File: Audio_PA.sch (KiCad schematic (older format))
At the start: 71 parts, among them P1 Audio_In, P2 TP, P3 TP, P4 +45VDC, P5 Audio_Out, P6 -45VDC, Q1 BCM856DS, Q10 2N3904, Q11 2N3906, Q12 IRFP240, Q13 IRFP9240, Q2 BCM856DS, Q3 MJE340, Q4 MJE350, Q5 MJE350, Q6 MJE340, Q7 BD139, Q8 MJE340, Q9 MJE350

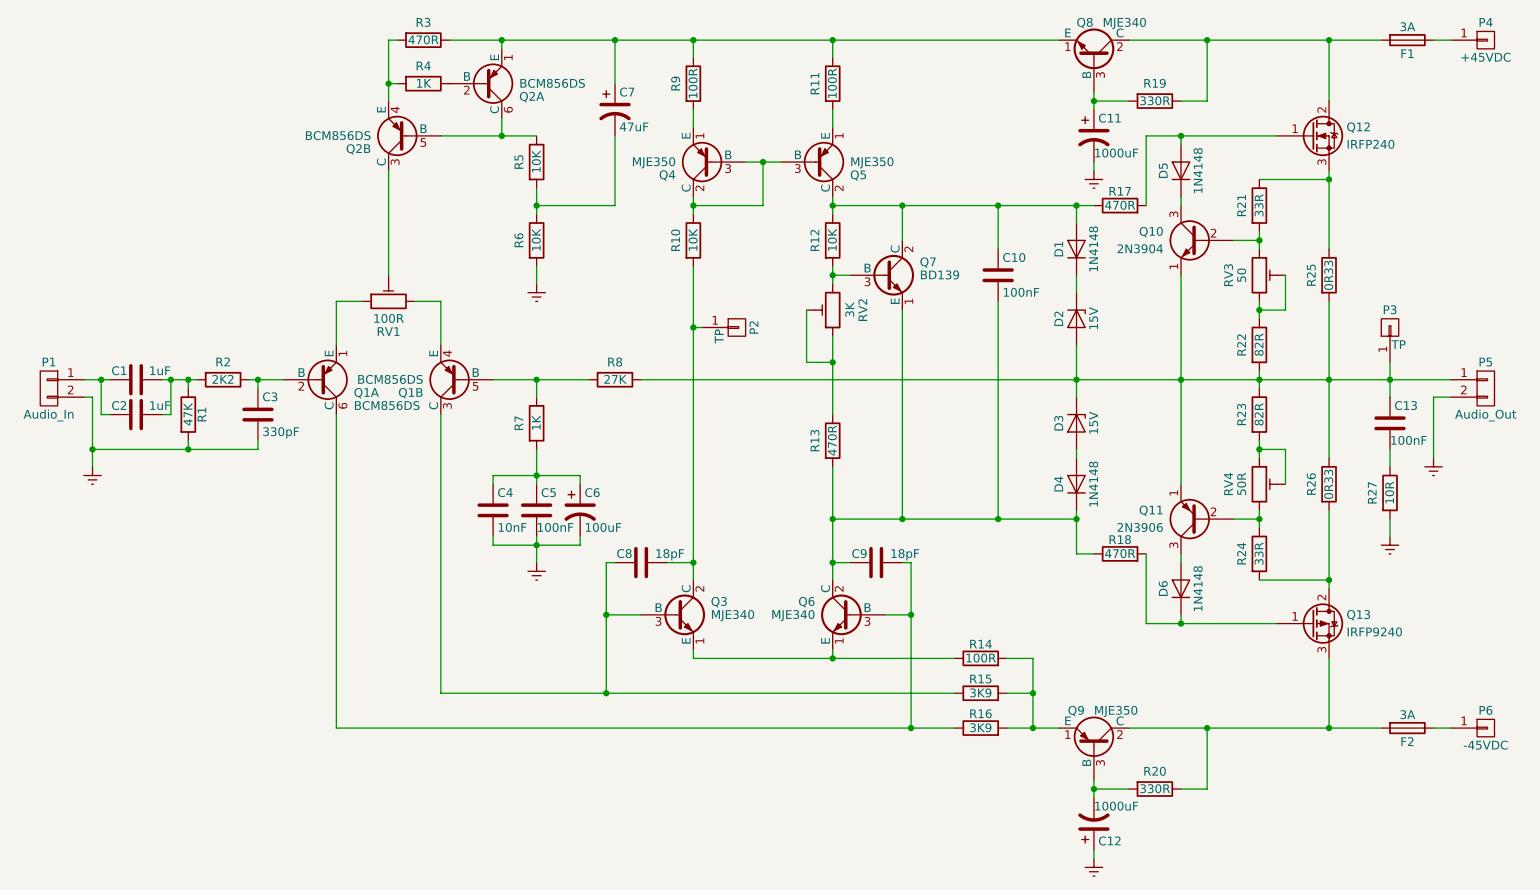
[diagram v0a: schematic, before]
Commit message: Layout V1 added
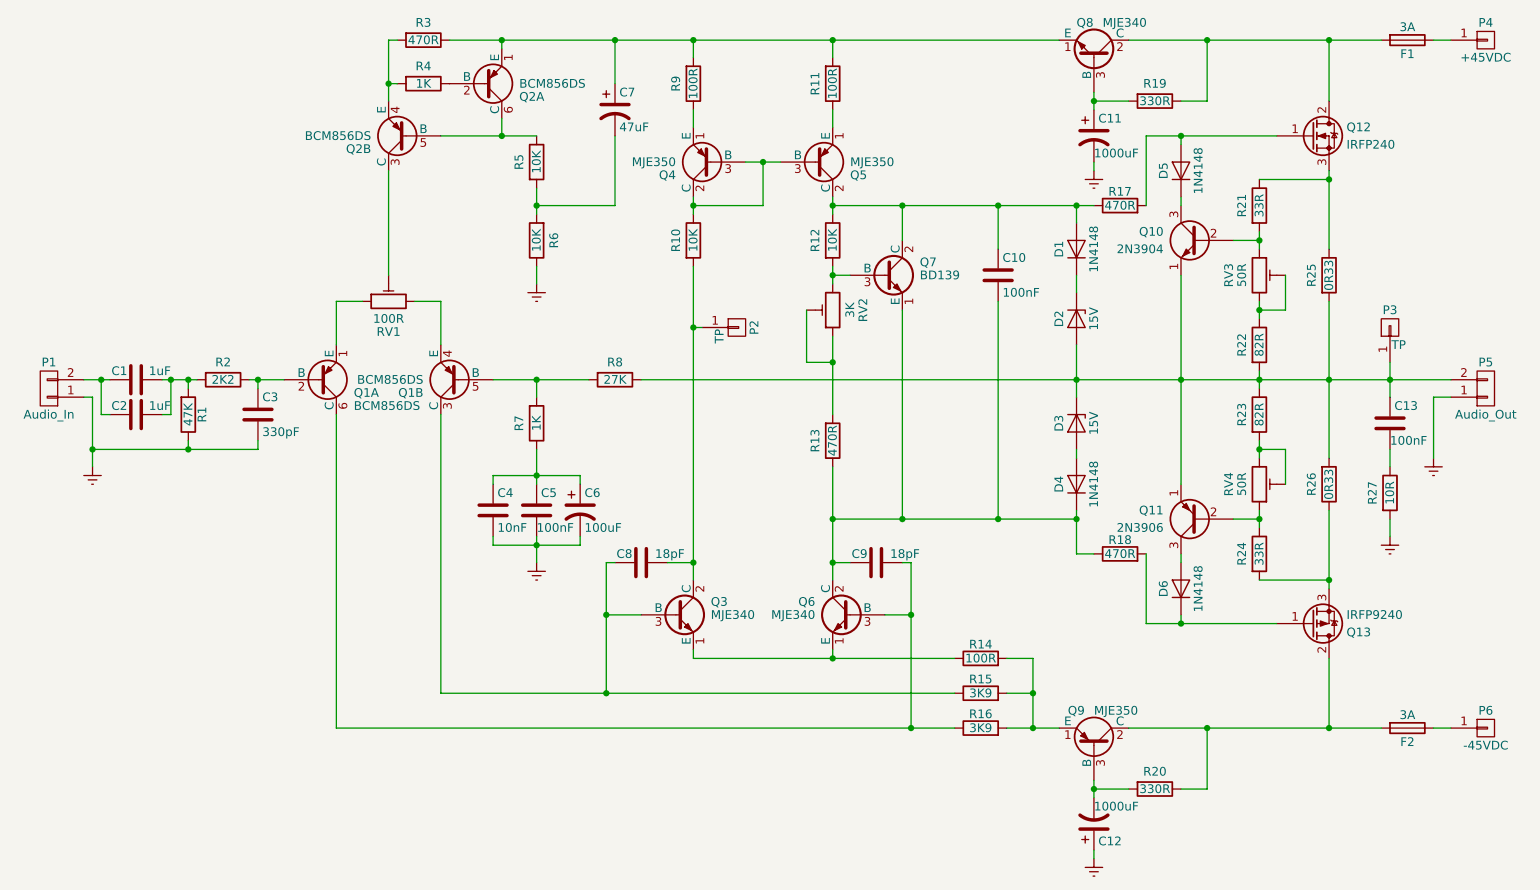
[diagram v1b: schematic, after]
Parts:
- Q7: footprint (none) -> TO_SOT_Packages_THT:SOT126_SOT32_Housing_Vertical
- RV3: value 50 -> 50R
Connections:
- net Earth: now also P1.1 (P1), P5.1 (P1), R1.1, R6.1; no longer P1.2 (P2), P5.2 (P2), R1.2, R6.2
- net at C1.1, C2.1: now also P1.2 (P2); no longer P1.1 (P1)
- net at C1.2, C2.2, R2.2: now also R1.2; no longer R1.1
- net at C7.1, Q2.1 (E), Q8.1 (E)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: now also R11.2, R9.2; no longer R11.1, R9.1
- net at Q1.5 (B), R8.2: now also R7.2; no longer R7.1
- net at C7.2, R5.2: now also R6.2; no longer R6.1
- net at Q4.1 (E): now also R9.1; no longer R9.2
- net at Q5.1 (E): now also R11.1; no longer R11.2
- net at C10.2, C9.1, D4.1 (K)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: now also R13.1; no longer R13.2
- net at C4.1, C5.1, C6.1: now also R7.1; no longer R7.2
- net at C13.1, D2.2 (A), D3.1 (K)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: now also P5.2 (P2), R26.2; no longer P5.1 (P1), R26.1
- net at F2.2, Q9.2 (C), R20.1: now also Q13.2 (D); no longer Q13.3 (S)
- net at RV2.1, RV2.2: now also R13.2; no longer R13.1
- net at Q11.2 (B), R24.1: now also RV4.1; no longer RV4.3
- net at R23.2, RV4.2: now also RV4.3; no longer RV4.1
- new net: Q13.3 (S), R24.2, R26.1
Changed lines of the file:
@@
 U 1 1 58727E75
 P 1150 3500
-F 0 "P1" H 1150 3650 50  0000 C CNN
-F 1 "Audio_In" H 1150 3350 50  0000 C CNN
+F 0 "P1" H 1150 3350 50  0000 C CNN
+F 1 "Audio_In" H 1150 3650 50  0000 C CNN
 F 2 "Connectors_Phoenix:PhoenixContact_MCV-G_02x3.81mm_Vertical" H 1150 3500 50  0001 C CNN
 F 3 "http://www.farnell.com/datasheets/2138215.pdf?_ga=1.58707370.1020810156.1482221903" H 1150 3500 50  0001 C CNN
 	1    1150 3500
-	-1   0    0    -1
+	-1   0    0    1
 $EndComp
 $Comp
@@
 F 3 "" H 1950 3650 50  0001 C CNN
 	1    1950 3650
-	1    0    0    -1
+	1    0    0    1
 $EndComp
 $Comp
@@
 $EndComp
 $Comp
-L Earth #PWR1
+L Earth #PWR01
 U 1 1 587282CB
 P 1400 3950
-F 0 "#PWR1" H 1400 3700 50  0001 C CNN
+F 0 "#PWR01" H 1400 3700 50  0001 C CNN
 F 1 "Earth" H 1400 3800 50  0001 C CNN
 F 2 "" H 1400 3950 50  0000 C CNN
@@
 F 3 "" H 3950 2650 50  0000 C CNN
 	1    3950 2650
-	1    0    0    -1
-$EndComp
-$Comp
-L Earth #PWR2
+	-1   0    0    1
+$EndComp
+$Comp
+L Earth #PWR02
 U 1 1 587293F8
 P 3950 2900
-F 0 "#PWR2" H 3950 2650 50  0001 C CNN
+F 0 "#PWR02" H 3950 2650 50  0001 C CNN
 F 1 "Earth" H 3950 2750 50  0001 C CNN
 F 2 "" H 3950 2900 50  0000 C CNN
@@
 F 3 "" H 4850 1750 50  0000 C CNN
 	1    4850 1750
-	1    0    0    -1
+	1    0    0    1
 $EndComp
 $Comp
@@
 F 3 "" H 5650 1750 50  0000 C CNN
 	1    5650 1750
-	1    0    0    -1
+	1    0    0    1
 $EndComp
 $Comp
@@
 F 3 "" H 3950 3700 50  0000 C CNN
 	1    3950 3700
-	1    0    0    -1
+	1    0    0    1
 $EndComp
 $Comp
@@
 $EndComp
 $Comp
-L Earth #PWR3
+L Earth #PWR03
 U 1 1 5872AAFE
 P 3950 4500
-F 0 "#PWR3" H 3950 4250 50  0001 C CNN
+F 0 "#PWR03" H 3950 4250 50  0001 C CNN
 F 1 "Earth" H 3950 4350 50  0001 C CNN
 F 2 "" H 3950 4500 50  0000 C CNN
@@
 U 1 1 5872E2CF
 P 9400 3500
-F 0 "P5" H 9400 3650 50  0000 C CNN
-F 1 "Audio_Out" H 9400 3350 50  0000 C CNN
+F 0 "P5" H 9400 3350 50  0000 C CNN
+F 1 "Audio_Out" H 9400 3650 50  0000 C CNN
 F 2 "Connectors_Phoenix:PhoenixContact_MCV-G_02x3.81mm_Vertical" H 9400 3500 50  0001 C CNN
 F 3 "" H 9400 3500 50  0000 C CNN
 	1    9400 3500
-	1    0    0    -1
-$EndComp
-$Comp
-L Earth #PWR7
+	1    0    0    1
+$EndComp
+$Comp
+L Earth #PWR04
 U 1 1 5872EA23
 P 9100 3900
-F 0 "#PWR7" H 9100 3650 50  0001 C CNN
+F 0 "#PWR04" H 9100 3650 50  0001 C CNN
 F 1 "Earth" H 9100 3750 50  0001 C CNN
 F 2 "" H 9100 3900 50  0000 C CNN
@@
 $EndComp
 $Comp
-L Earth #PWR6
+L Earth #PWR05
 U 1 1 5872FA97
 P 8850 4350
-F 0 "#PWR6" H 8850 4100 50  0001 C CNN
+F 0 "#PWR05" H 8850 4100 50  0001 C CNN
 F 1 "Earth" H 8850 4200 50  0001 C CNN
 F 2 "" H 8850 4350 50  0000 C CNN
@@
 F 3 "" H 5650 3800 50  0000 C CNN
 	1    5650 3800
-	1    0    0    -1
+	1    0    0    1
 $EndComp
 $Comp
@@
 F 0 "Q7" H 6150 2925 50  0000 L CNN
 F 1 "BD139" H 6150 2850 50  0000 L CNN
-F 2 "" H 6150 2775 50  0000 L CIN
+F 2 "TO_SOT_Packages_THT:SOT126_SOT32_Housing_Vertical" H 6150 2775 50  0001 L CIN
 F 3 "" H 5950 2850 50  0000 L CNN
 	1    5950 2850
@@
 F 4 ">=5W" V 8500 4050 60  0001 C CNN "Wattage"
 	1    8500 4050
-	1    0    0    -1
+	1    0    0    1
 $EndComp
 $Comp
@@
 F 3 "" H 8400 4850 50  0000 C CNN
 	1    8400 4850
-	1    0    0    -1
+	1    0    0    1
 $EndComp
 $Comp
@@
 $EndComp
 $Comp
-L Earth #PWR4
+L Earth #PWR06
 U 1 1 5875481E
 P 7150 2250
-F 0 "#PWR4" H 7150 2000 50  0001 C CNN
+F 0 "#PWR06" H 7150 2000 50  0001 C CNN
 F 1 "Earth" H 7150 2100 50  0001 C CNN
 F 2 "" H 7150 2250 50  0000 C CNN
@@
 $EndComp
 $Comp
-L Earth #PWR5
+L Earth #PWR07
 U 1 1 587571E8
 P 7150 6200
-F 0 "#PWR5" H 7150 5950 50  0001 C CNN
+F 0 "#PWR07" H 7150 5950 50  0001 C CNN
 F 1 "Earth" H 7150 6050 50  0001 C CNN
 F 2 "" H 7150 6200 50  0000 C CNN
@@
 P 8100 2850
 F 0 "RV3" V 7925 2850 50  0000 C CNN
-F 1 "50" V 8000 2850 50  0000 C CNN
+F 1 "50R" V 8000 2850 50  0000 C CNN
 F 2 "Potentiometers:Potentiometer_Bourns_3296Y_3-8Zoll_Angular_ScrewUp" H 8100 2850 50  0001 C CNN
 F 3 "http://www.farnell.com/datasheets/2061261.pdf?_ga=1.94292381.1020810156.1482221903" H 8100 2850 50  0001 C CNN
@@
 F 4 "Multi Turn" V 8100 4050 60  0001 C CNN "Type"
 	1    8100 4050
-	1    0    0    -1
+	1    0    0    1
 $EndComp
 Wire Wire Line
